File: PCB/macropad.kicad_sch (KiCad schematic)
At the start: 33 parts, among them SW1 SW_Push, SW10 SW_Push, SW11 SW_Push, SW12 SW_Push, SW13 SW_Push, SW14 SW_Push, SW15 SW_Push, SW16 SW_Push, SW2 SW_Push, SW3 SW_Push, SW4 SW_Push, SW5 SW_Push, SW6 SW_Push, SW7 SW_Push, SW8 SW_Push, SW9 SW_Push, U1 Seeed Studio XIAO SAMD21

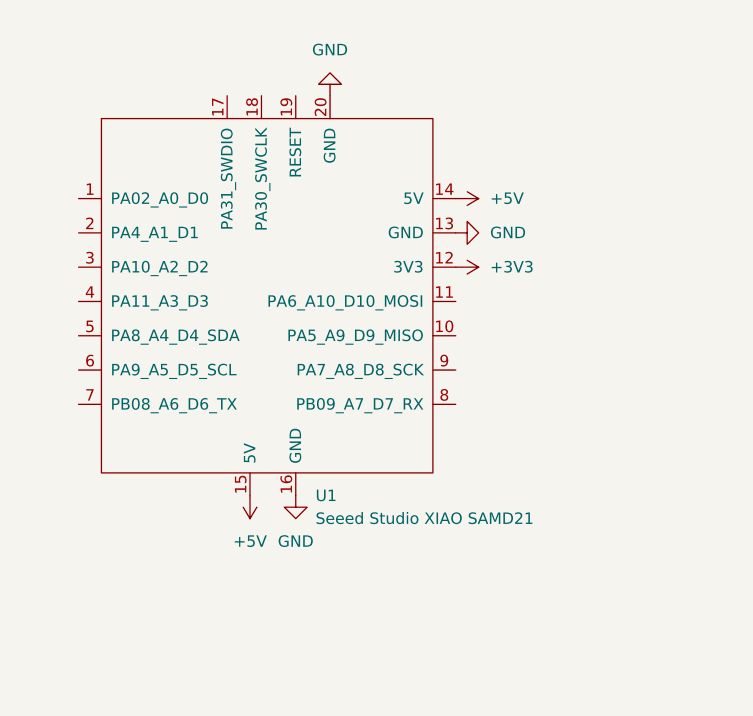
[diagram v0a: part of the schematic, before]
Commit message: Finish first state of PCB
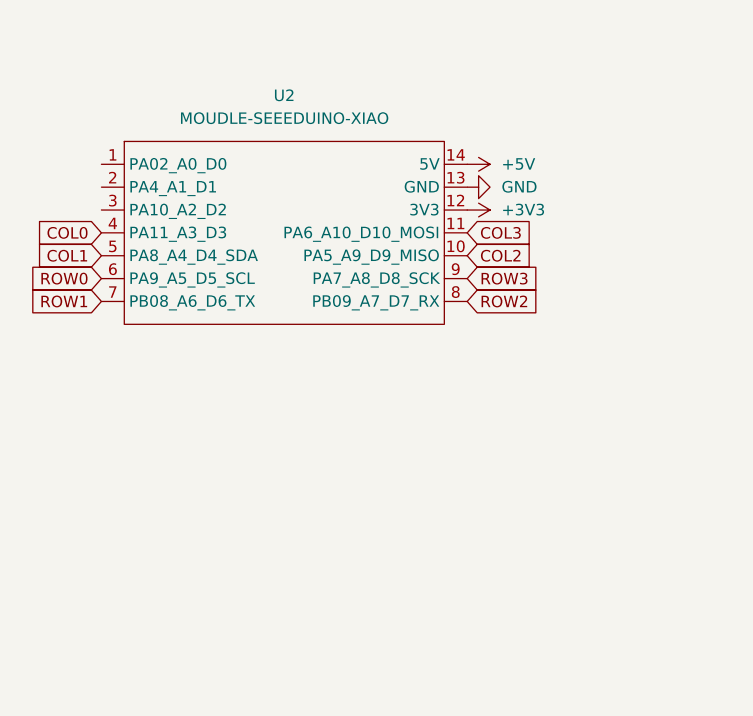
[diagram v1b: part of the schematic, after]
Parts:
- removed U1: Seeed Studio XIAO SAMD21, seed:XIAO-SAMD21-RP2040-14P-2.54-21X17.8MM (Seeeduino XIAO), symbol seed:Seeed Studio XIAO SAMD21
- added U2: MOUDLE-SEEEDUINO-XIAO, seed:XIAO-SAMD21-RP2040-14P-2.54-21X17.8MM (Seeeduino XIAO), symbol seed-real:MOUDLE-SEEEDUINO-XIAO
- D1, D10, D11, D12, D13, D14, D15, D16, D2, D3, D4, D5, D6, D7, D8, D9: footprint Diode_THT:D_5KP_P10.16mm_Horizontal -> Diode_THT:D_DO-35_SOD27_P7.62mm_Horizontal
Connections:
- net +3V3: now also U2.12 (3V3)
- net +5V: now also U2.14 (5V)
- net COL0: now also U2.4 (PA11_A3_D3)
- net COL1: now also U2.5 (PA8_A4_D4_SDA)
- net COL2: now also U2.10 (PA5_A9_D9_MISO)
- net COL3: now also U2.11 (PA6_A10_D10_MOSI)
- net GND: now also U2.13 (GND)
- net ROW0: now also U2.6 (PA9_A5_D5_SCL)
- net ROW1: now also U2.7 (PB08_A6_D6_TX)
- net ROW2: now also U2.8 (PB09_A7_D7_RX)
- net ROW3: now also U2.9 (PA7_A8_D8_SCK)

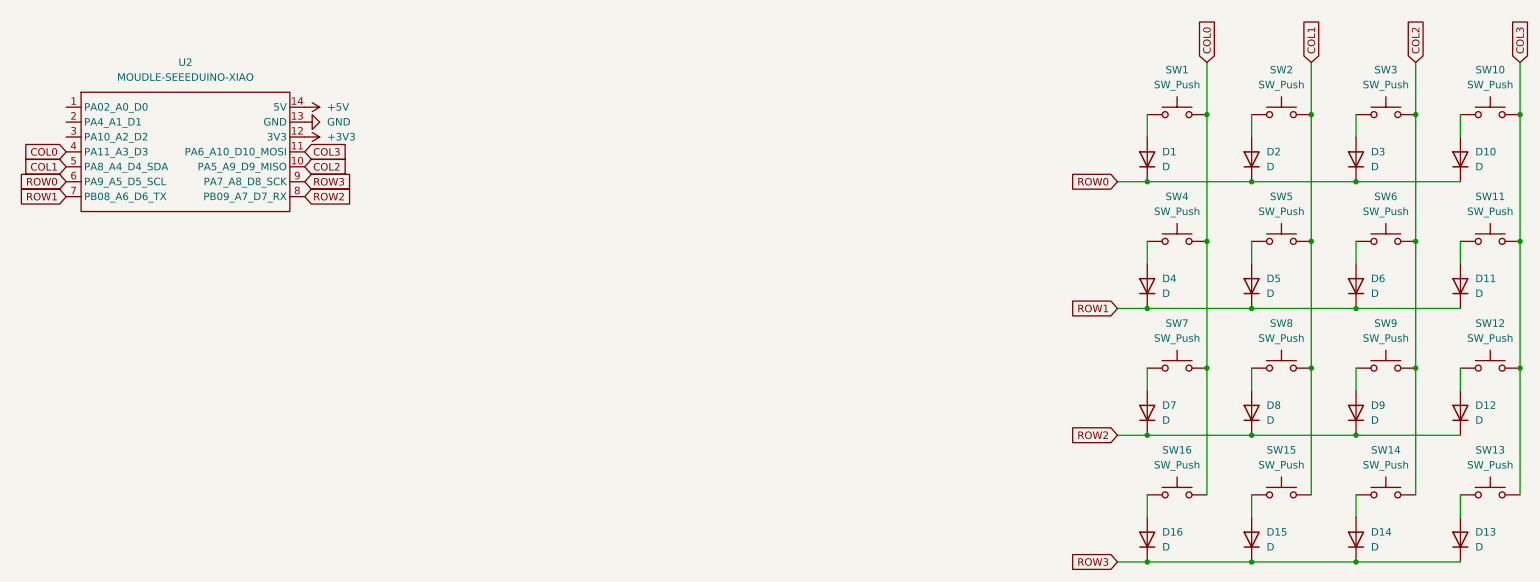
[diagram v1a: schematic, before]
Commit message: LCD!
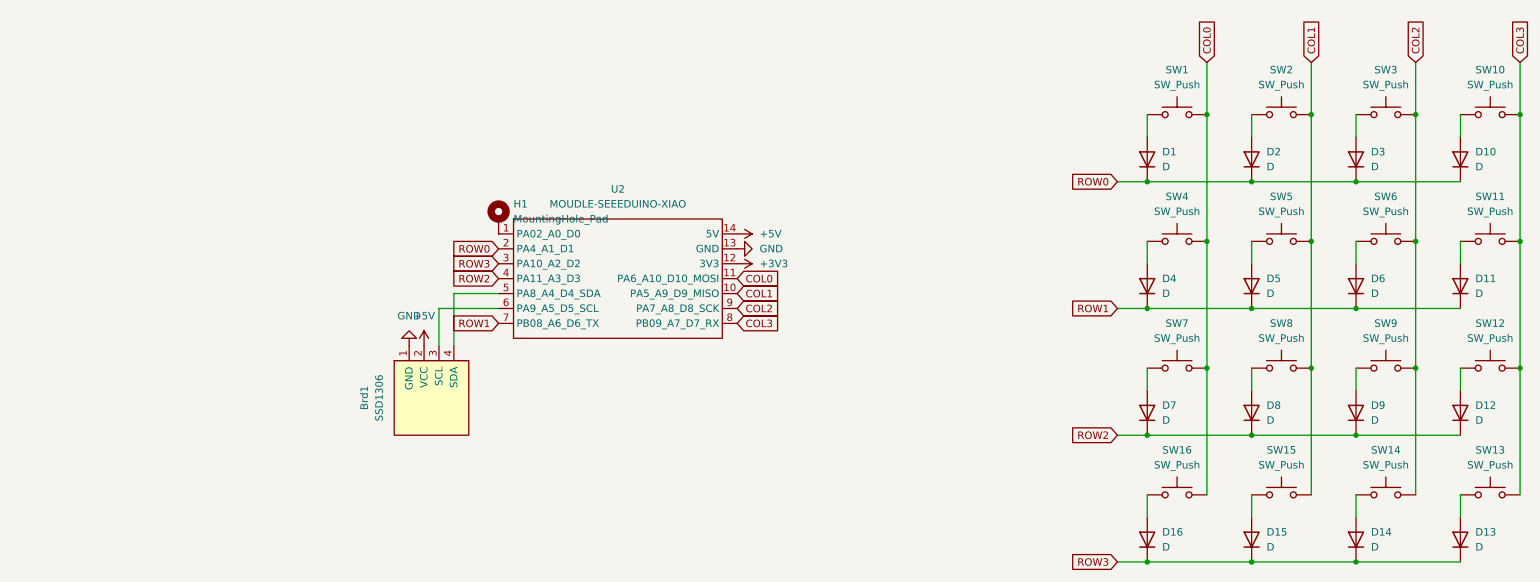
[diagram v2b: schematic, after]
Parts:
- added Brd1: SSD1306, screen:128x64OLED, symbol screen:SSD1306
- added H1: MountingHole_Pad, Connector_Wire:SolderWire-0.1sqmm_1x01_D0.4mm_OD1mm, symbol Mechanical:MountingHole_Pad
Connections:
- net +5V: now also Brd1.2 (VCC)
- net COL0: now also U2.11 (PA6_A10_D10_MOSI); no longer U2.4 (PA11_A3_D3)
- net COL1: now also U2.10 (PA5_A9_D9_MISO); no longer U2.5 (PA8_A4_D4_SDA)
- net COL2: now also U2.9 (PA7_A8_D8_SCK); no longer U2.10 (PA5_A9_D9_MISO)
- net COL3: now also U2.8 (PB09_A7_D7_RX); no longer U2.11 (PA6_A10_D10_MOSI)
- net GND: now also Brd1.1 (GND)
- net ROW0: now also U2.2 (PA4_A1_D1); no longer U2.6 (PA9_A5_D5_SCL)
- net ROW2: now also U2.4 (PA11_A3_D3); no longer U2.8 (PB09_A7_D7_RX)
- net ROW3: now also U2.3 (PA10_A2_D2); no longer U2.9 (PA7_A8_D8_SCK)
- net at U2.1 (PA02_A0_D0): now also H1.1
- new net: Brd1.4 (SDA), U2.5 (PA8_A4_D4_SDA)
- new net: Brd1.3 (SCL), U2.6 (PA9_A5_D5_SCL)
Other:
- moved on the sheet: U2
